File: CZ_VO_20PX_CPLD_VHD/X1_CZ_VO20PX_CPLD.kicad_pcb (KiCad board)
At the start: 2 copper layers, 137 x 140 mm, 112 parts, among them IC1 EMP7064_PLCC84, IC10 4538, IC100 ATmega328P-PU, IC101 ATmega328P-PU, IC102 4069, IC11 4013, IC120 LM1881, IC2 8251, IC3 74LS245, IC4 74LS393, IC5 74LS541, IC7 74LS02, IC8 74LS688, J1 CONN_01x05, J2 CONN_01x05, J3 DB15_Female_MountingHoles, J4 AVR-JTAG-10, M1 CONN_01x01, M1_F1 CONN_01x01, Q2 NPN (D637) or BC635, SW1 CONN_02x04, SW2 CONN_02x05, SW3 CONN_02x08, X1 CXO_DIP8, Y1 16Mhz, Y2 16Mhz

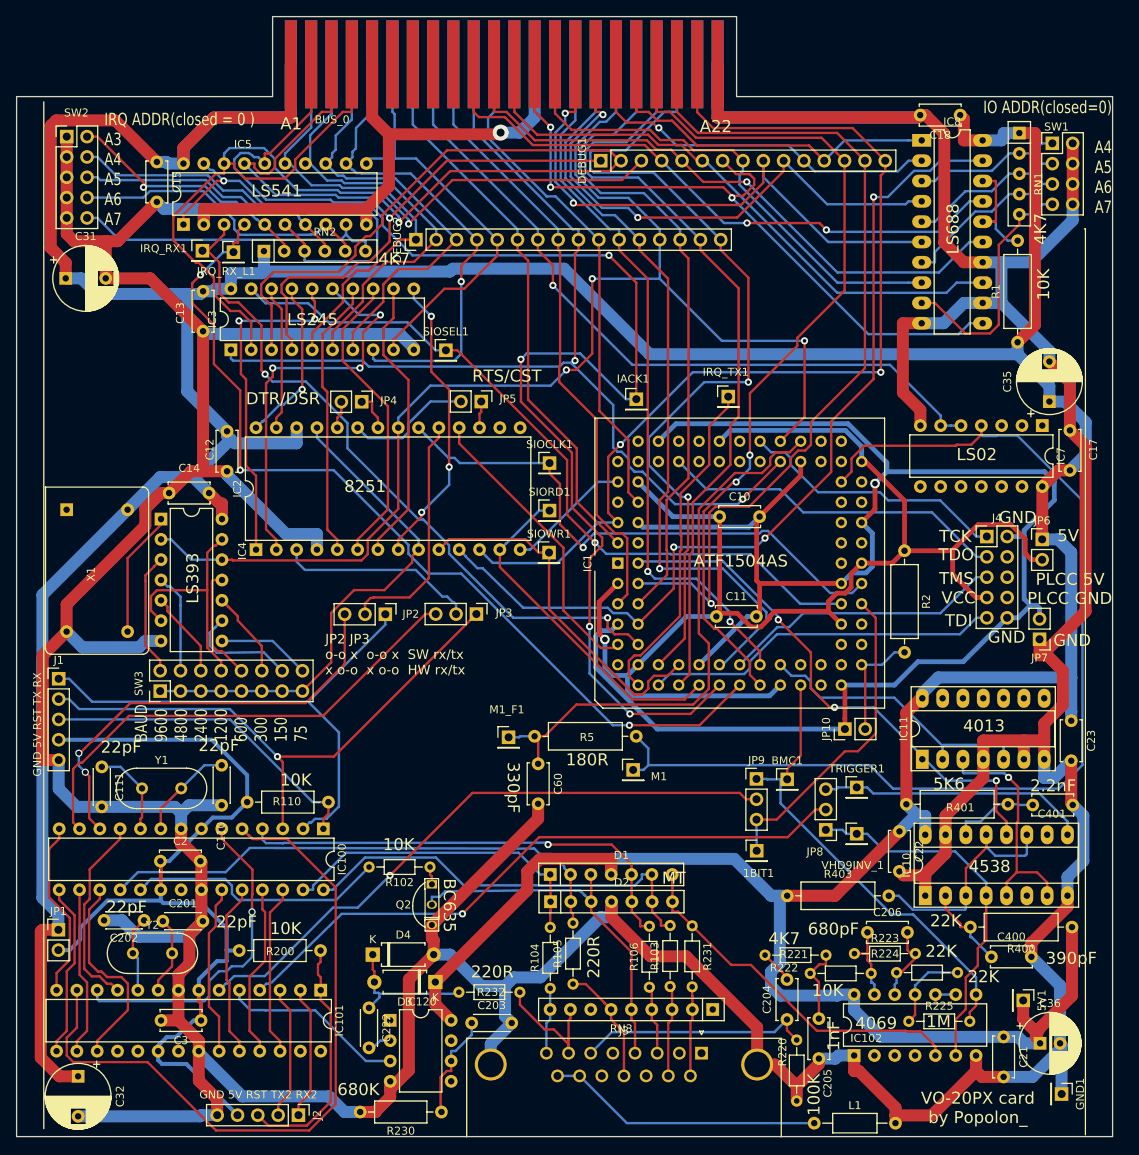
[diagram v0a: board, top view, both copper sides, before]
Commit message: Add files via upload
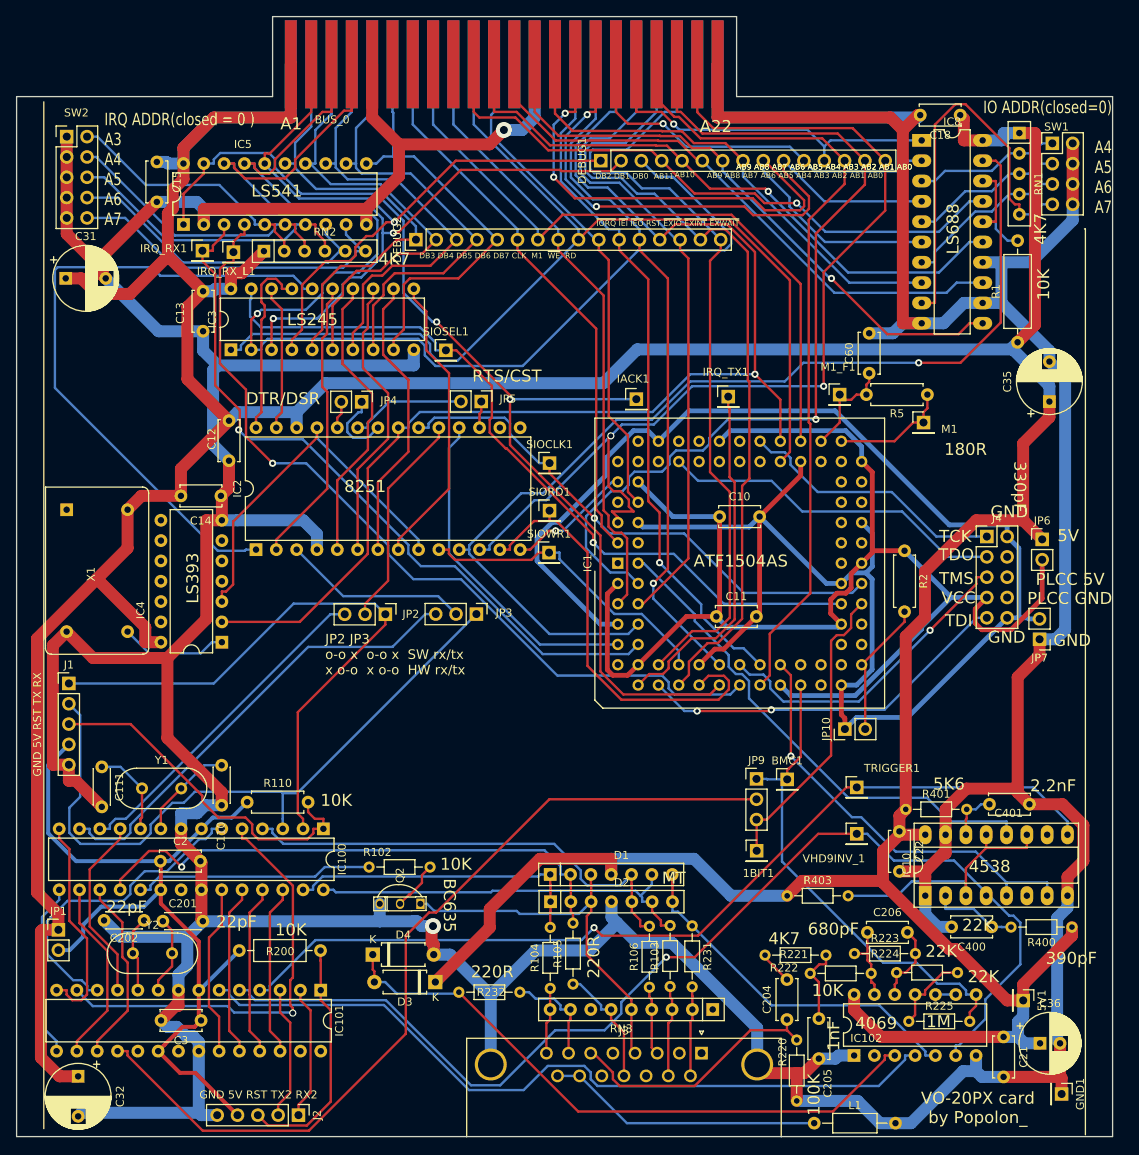
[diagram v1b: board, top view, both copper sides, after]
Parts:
- removed C17, C23: 100nF, Capacitor_THT:C_Disc_D5.0mm_W2.5mm_P5.00mm
- removed C203, C222: 100nF, Capacitor_THT:C_Disc_D4.3mm_W1.9mm_P5.00mm
- removed IC11: 4013, Package_DIP:DIP-14_W7.62mm_Socket_LongPads
- removed IC120: LM1881, Package_DIP:DIP-8_W7.62mm
- removed IC7: 74LS02, Package_DIP:DIP-14_W7.62mm
- removed JP8: Jumper_3_Open, Connector_PinHeader_2.54mm:PinHeader_1x03_P2.54mm_Vertical
- removed R230: 680K, Resistor_THT:R_Axial_DIN0207_L6.3mm_D2.5mm_P10.16mm_Horizontal
- removed SW3: CONN_02x08, Connector_PinHeader_2.54mm:PinHeader_2x08_P2.54mm_Vertical
- Q2: value NPN (D637) or BC635 -> NPN (BC546)
- R110: footprint Resistor_THT:R_Axial_DIN0207_L6.3mm_D2.5mm_P10.16mm_Horizontal -> Resistor_THT:R_Axial_DIN0207_L6.3mm_D2.5mm_P7.62mm_Horizontal
- R2, R5: footprint Resistor_THT:R_Axial_DIN0309_L9.0mm_D3.2mm_P12.70mm_Horizontal -> Resistor_THT:R_Axial_DIN0207_L6.3mm_D2.5mm_P7.62mm_Horizontal
- R400, R401, R403: footprint Resistor_THT:R_Axial_DIN0309_L9.0mm_D3.2mm_P12.70mm_Horizontal -> Resistor_THT:R_Axial_DIN0204_L3.6mm_D1.6mm_P7.62mm_Horizontal
- moved C60 64.0 mm to (234.6, 137.6), turned to 90 degrees
- moved M1_F1 59.6 mm to (230.9, 140.3)
- moved M1 56.6 mm to (241.4, 143.8)
- moved R5 56.1 mm to (241.9, 140.3)
- moved IC4 17.2 mm to (153.7, 171.2), turned to 180 degrees
- moved C401 5.41 mm to (249.6, 191.5)
- moved C400 3.75 mm to (249.9, 206.8), turned to 180 degrees
- moved C14 3.53 mm to (148.6, 152.9), turned to 0 degrees
- moved Q2 2.83 mm to (178.5, 203.9), turned to 180 degrees
- moved J1 1.40 mm to (134.6, 176.4)
- moved C12 1.34 mm to (154.6, 143.5)
- moved R401 0.64 mm to (239.2, 192.1)
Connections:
- D3 pad 2: Net-(C222-Pad1) -> Net-(D3-Pad2)
- D4 pad 1: Net-(C222-Pad1) -> Net-(D3-Pad2)
- IC1 pad 52: M1 -> (no net)
- IC1 pad 54: (no net) -> M1
- IC1 pad 56: (no net) -> M1_FILTERED
- IC1 pad 58: M1_FILTERED -> ~M1
- IC10 pad 4: VHD9_INV -> ~VHD9_PACKET_SYNC
- IC10 pad 5: Net-(IC10-Pad5) -> DCLK1
- IC10 pad 7: Net-(IC10-Pad5) -> DCLK1
- IC101 pad 18: (no net) -> Net-(IC101-Pad18)
- IC101 pad 4: Net-(IC101-Pad4) -> VHD_1BIT_TRIGGER
- IC101 pad 5: V_SYNCH -> ~VHD9_PACKET_SYNC
- IC101 pad 6: Net-(IC101-Pad6) -> ~COMPOSITE_SYNCH
- IC102 pad 3: (no net) -> Net-(D3-Pad2)
- IC102 pad 4: (no net) -> ~COMPOSITE_SYNCH
- IC102 pad 6: VHD9_INV -> ~VHD9_PACKET_SYNC
- IC4 pad 10: Net-(IC4-Pad10) -> (no net)
- IC4 pad 11: Net-(IC4-Pad11) -> (no net)
- IC4 pad 12: RESET -> (no net)
- IC4 pad 13: Net-(IC4-Pad13) -> (no net)
- IC4 pad 3: Net-(IC4-Pad3) -> TxRxCLK
- IC4 pad 4: Net-(IC4-Pad4) -> (no net)
- IC4 pad 5: Net-(IC4-Pad5) -> (no net)
- IC4 pad 6: Net-(IC4-Pad13) -> (no net)
- IC4 pad 8: Net-(IC4-Pad8) -> (no net)
- IC4 pad 9: Net-(IC4-Pad9) -> (no net)
- JP9 pad 2: Net-(IC101-Pad6) -> Net-(IC101-Pad18)
- Q2 pad 1: Net-(Q2-Pad1) -> VHD4
- Q2 pad 2: VHD4 -> Net-(Q2-Pad2)
- R102 pad 1: Net-(Q2-Pad1) -> Net-(Q2-Pad2)
- R232 pad 1: Net-(C222-Pad1) -> Net-(D3-Pad2)
- VHD9INV_1 pad 1: VHD9_INV -> ~VHD9_PACKET_SYNC
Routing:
- net ~VHD9_PACKET_SYNC: track 0.00 -> 141.9 mm, vias 0 -> 1
- net M1: track 135.4 -> 14.9 mm
- net Net-(IC101-Pad18): track 0.00 -> 108.7 mm
- net ~COMPOSITE_SYNCH: track 0.00 -> 97.2 mm
- net VHD_1BIT_TRIGGER: track 33.7 -> 116.0 mm, vias 0 -> 1
- net Net-(IC101-Pad4): track 80.1 -> 0.00 mm, vias 1 -> 0
- net Net-(D3-Pad2): track 0.00 -> 78.6 mm
- net Net-(IC101-Pad6): track 77.7 -> 0.00 mm, vias 1 -> 0
- net M1_FILTERED: track 70.7 -> 13.2 mm
- net GND: track 850.5 -> 794.5 mm, vias 1 -> 2
- net VHD9_INV: track 46.0 -> 0.00 mm
- net 5V: track 643.3 -> 597.7 mm
- net DB0: track 120.4 -> 162.7 mm
- net Net-(IC2-Pad1): track 43.0 -> 82.1 mm, vias 2 -> 0
- net DB1: track 137.6 -> 101.8 mm, vias 1 -> 2
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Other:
- board text added: "AB10"
- board text added: "AB11"
- board text added: "AB9 AB8 AB7 AB6 AB5 AB4 AB3 AB2 AB1 AB0"
- board text added: "DB2 DB1 DB0"
- board text added: "DB3 DB4 DB5 DB6 DB7 CLK M1 ~WE~ RD"
- board text added: "~IORQ~ ~IEI~ ~IEO~ RST ~EXIO~ ~EXINT~ ~EXWAIT"
- board text removed: "4013"
- board text removed: "680K"
- board text removed: "BAUD 9600 4800 2400 1200 600 300 150 75"
- board text removed: "LS02"
